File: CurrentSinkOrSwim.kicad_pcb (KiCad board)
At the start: 2 copper layers, 41.7 x 38.9 mm, 25 parts, among them P1 CONN_01X01, P101 ext pwr, P102 pwr select, P103 Input, P2 V, P3 A, P4 Gnd, Q401 BUK9575, U201 LMV358, U301 LM2931D-R

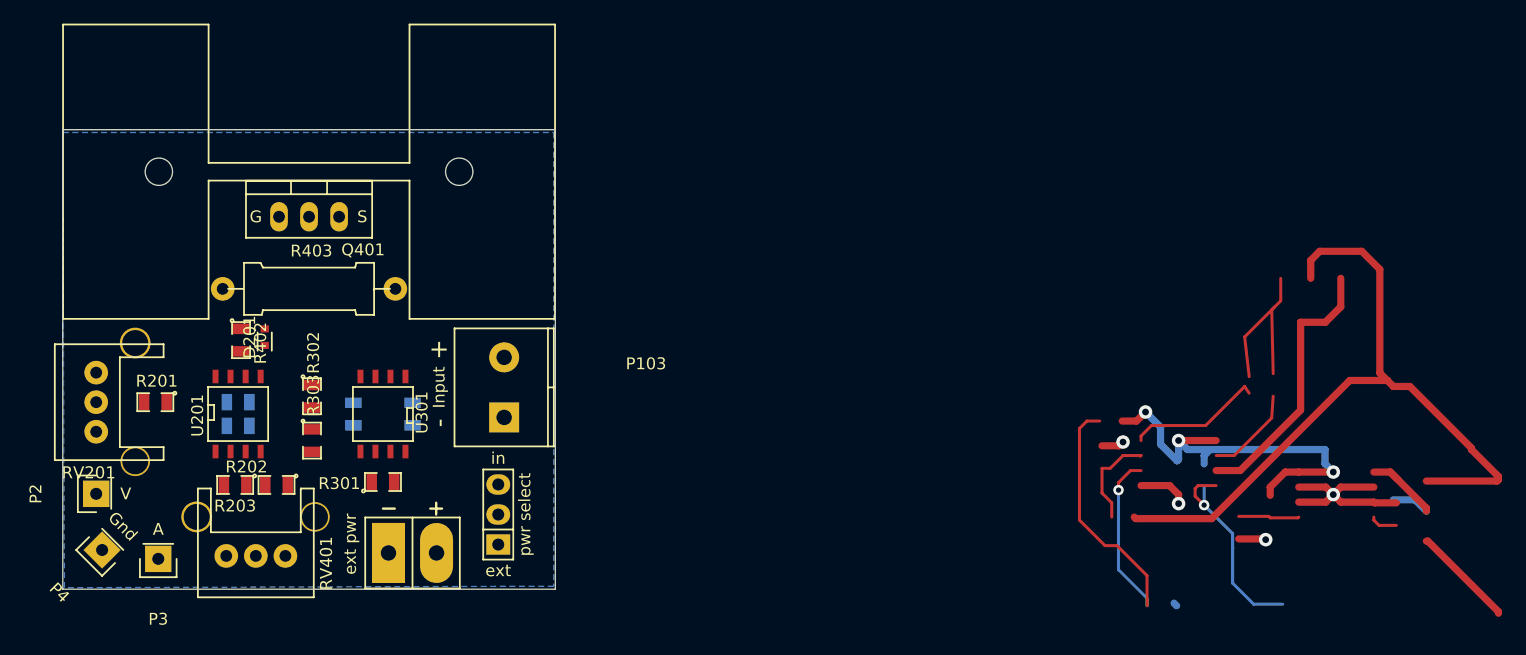
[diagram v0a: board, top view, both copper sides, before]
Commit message: Routing done
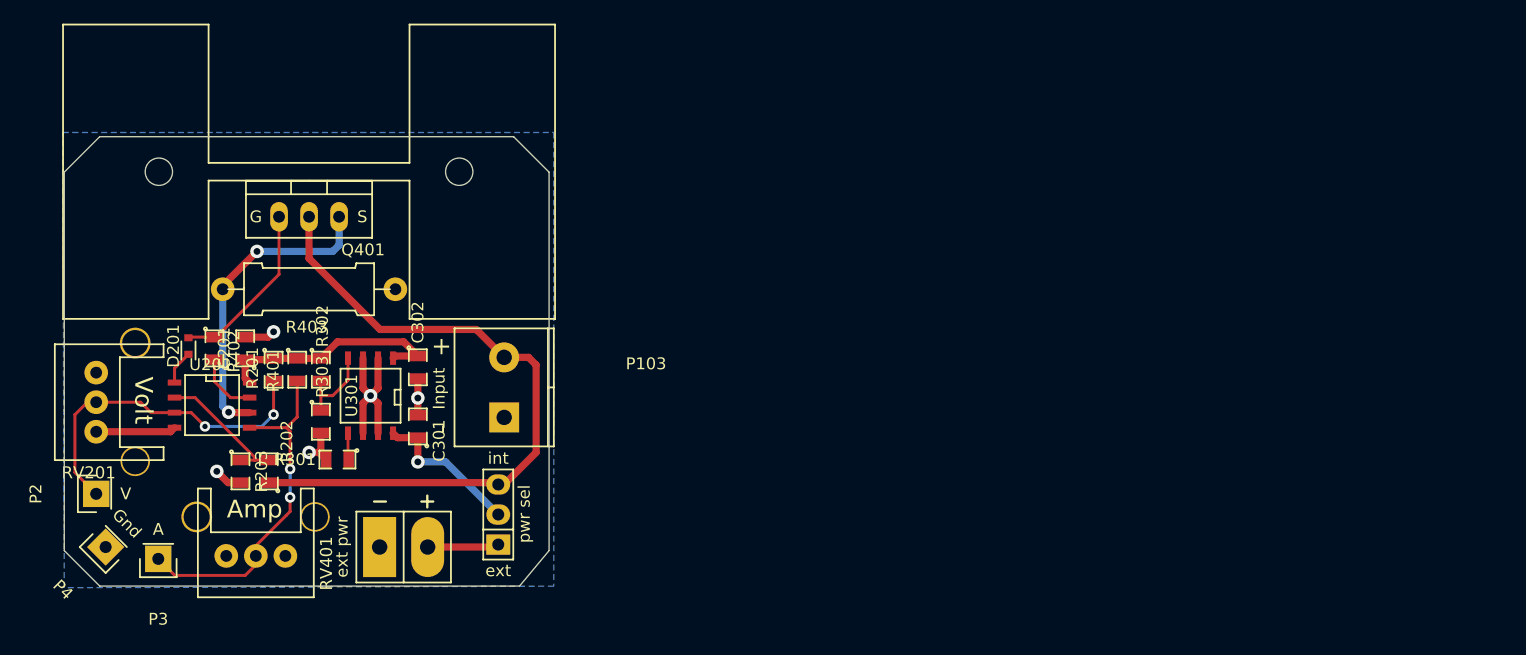
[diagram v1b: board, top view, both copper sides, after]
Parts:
- C201, C301, C302, R401: moved to F.Cu
- P101: footprint Current:Pads-01x02 -> Pads-01x02
- P102: value pwr select -> pwr sel
- moved R201 10.4 mm to (124.0, 65.0), turned to 270 degrees
- moved C302 6.73 mm to (136.2, 64.8), turned to 270 degrees
- moved C201 6.58 mm to (121.6, 63.2), turned to 90 degrees
- moved D201 6.49 mm to (116.8, 63.0)
- moved R401 5.71 mm to (126.0, 65.0), turned to 270 degrees
- moved R301 4.29 mm to (129.4, 72.6), turned to 180 degrees
- moved R302 2.37 mm to (128.0, 65.0)
- moved R402 2.36 mm to (119.0, 63.2)
- moved U201 2.32 mm to (118.8, 68.0), turned to 270 degrees
- moved U301 1.87 mm to (132.2, 67.2)
- moved R303 1.77 mm to (128.0, 69.4)
- moved R202 1.32 mm to (123.6, 73.6), turned to 90 degrees
- moved R203 1.23 mm to (121.2, 73.6), turned to 270 degrees
- moved C301 1.14 mm to (136.2, 69.8)
- moved P101 0.90 mm to (135.0, 80.0)
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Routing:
- net (no net): track 267.2 -> 0.00 mm, vias 9 -> 0
- net /Current Control/Current_Sink+: track 0.00 -> 57.6 mm
- net GND: track 0.00 -> 33.3 mm, vias 0 -> 5
- net Net-(P3-Pad1): track 0.00 -> 29.6 mm, vias 0 -> 2
- net Net-(P2-Pad1): track 0.00 -> 28.8 mm, vias 0 -> 2
- net Net-(Q401-PadS): track 0.00 -> 26.4 mm, vias 0 -> 2
- net 2.7V: track 0.00 -> 20.1 mm
- net /Current Control/FET_Gate: track 0.00 -> 15.1 mm
- net /Power Regulation/Vin: track 0.00 -> 12.9 mm, vias 0 -> 1
- net Net-(R202-Pad2): track 0.00 -> 11.5 mm
- net Net-(R302-Pad2): track 0.00 -> 7.21 mm
- net Net-(P101-Pad2): track 0.00 -> 6.05 mm
- net Net-(R402-Pad2): track 0.00 -> 5.39 mm
- net Net-(D201-Pad2): track 0.00 -> 2.88 mm
- net Net-(R301-Pad1): track 0.00 -> 2.25 mm
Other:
- board size 41.7 x 38.9 mm -> 41 x 38 mm
- board text added: "Amp"
- board text added: "Volt"
- board text added: "int"
- board text removed: "in"
